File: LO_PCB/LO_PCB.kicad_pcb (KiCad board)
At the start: 4 copper layers, 50 x 44 mm, 97 parts, among them J1 PWR, J2 Conn_01x06, Q1 AO3401A, U1 TPS7A9101DSKT, U2 LMX2582RHAR, X1 TB612-100.0M

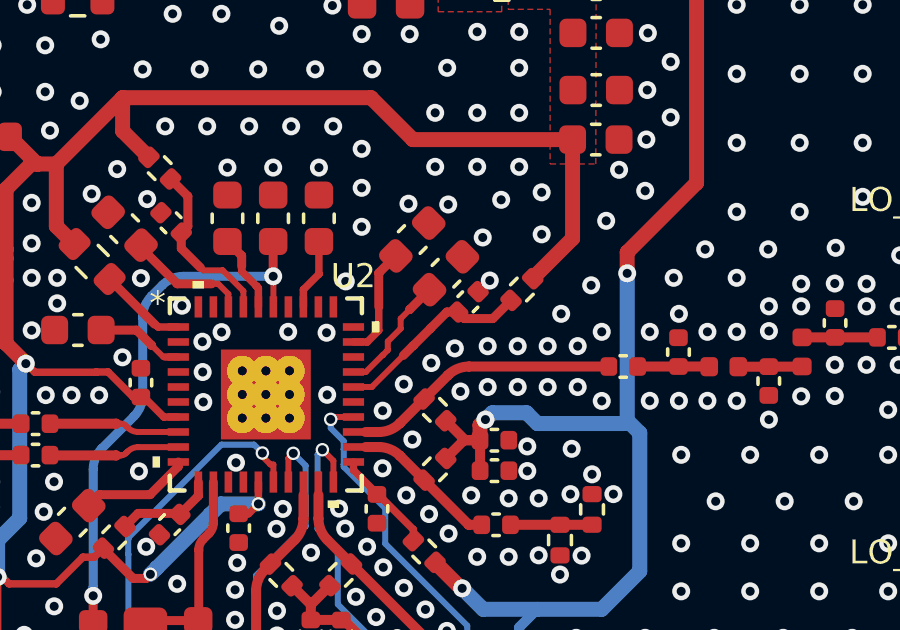
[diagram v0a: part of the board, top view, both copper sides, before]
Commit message: fixed errors and small bugs
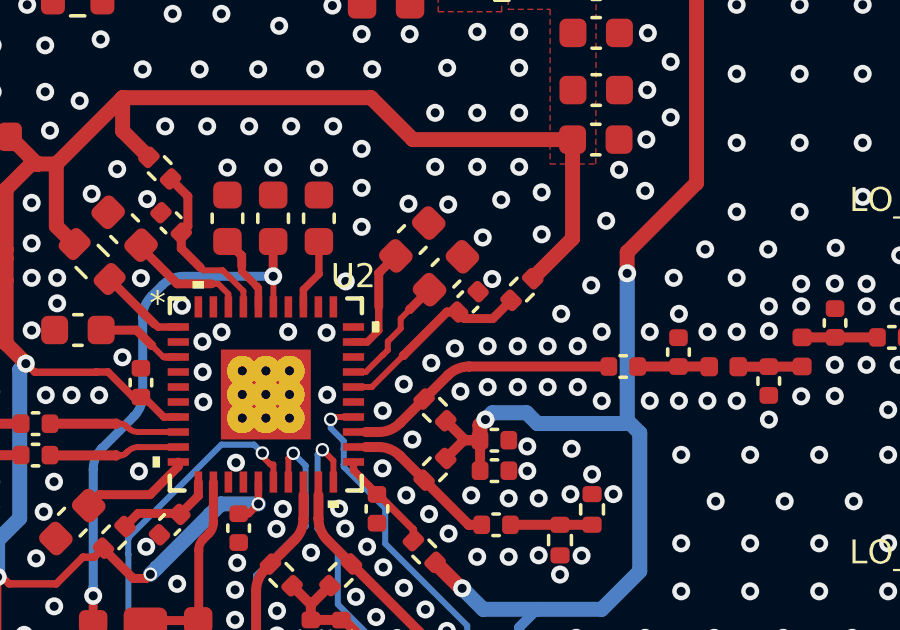
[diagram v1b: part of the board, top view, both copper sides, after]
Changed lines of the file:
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@@
 	)
 	(via
-		(at 165.02 94.69)
+		(at 165.1 94.6404)
 		(size 0.6)
 		(drill 0.3)
@@
 	)
 	(segment
-		(start 162.35 95.657092)
-		(end 163.011992 94.9951)
-		(width 0.3)
-		(layer "F.Cu")
-		(net "Net-(U2-VBIASVCO2)")
-	)
-	(segment
-		(start 162.05 96.292092)
-		(end 161.62 96.722092)
+		(start 161.62 97.01)
+		(end 161.455 97.175)
 		(width 0.2)
 		(layer "F.Cu")
@@
 	)
 	(segment
-		(start 160.886201 97.738799)
-		(end 160.476201 97.738799)
+		(start 161.45 97.175)
+		(end 160.886201 97.738799)
 		(width 0.2)
 		(layer "F.Cu")
@@
 	)
 	(segment
-		(start 161.62 97.01)
-		(end 161.455 97.175)
-		(width 0.2)
+		(start 162.35 95.66)
+		(end 162.35 95.657092)
+		(width 0.3)
 		(layer "F.Cu")
 		(net "Net-(U2-VBIASVCO2)")
 	)
 	(segment
-		(start 163.168446 95.1651)
-		(end 163.176992 95.1651)
-		(width 0.25)
+		(start 162.05 96.292092)
+		(end 161.62 96.722092)
+		(width 0.2)
 		(layer "F.Cu")
 		(net "Net-(U2-VBIASVCO2)")
 	)
 	(segment
-		(start 162.35 95.65)
-		(end 162.35 95.66)
+		(start 160.886201 97.738799)
+		(end 160.476201 97.738799)
 		(width 0.2)
 		(layer "F.Cu")
@@
 	)
 	(segment
-		(start 163.153982 95.1401)
-		(end 163.130621 95.1401)
+		(start 163.168446 95.1651)
+		(end 163.176992 95.1651)
 		(width 0.25)
 		(layer "F.Cu")
@@
 	)
 	(segment
-		(start 161.62 96.722092)
-		(end 161.62 97.01)
-		(width 0.2)
+		(start 163.153982 95.1401)
+		(end 163.130621 95.1401)
+		(width 0.25)
 		(layer "F.Cu")
 		(net "Net-(U2-VBIASVCO2)")
 	)
 	(segment
-		(start 162.35 95.66)
-		(end 162.35 95.657092)
+		(start 162.35 95.657092)
+		(end 163.011992 94.9951)
 		(width 0.3)
 		(layer "F.Cu")
@@
 	)
 	(segment
-		(start 162.05 95.96)
-		(end 162.05 96.292092)
+		(start 161.62 96.722092)
+		(end 161.62 97.01)
 		(width 0.2)
 		(layer "F.Cu")
@@
 	)
 	(segment
-		(start 161.45 97.175)
-		(end 160.886201 97.738799)
+		(start 162.05 95.96)
+		(end 162.05 96.292092)
 		(width 0.2)
 		(layer "F.Cu")
@@
 	)
 	(segment
-		(start 162.138117 97.188117)
-		(end 162.461335 96.8649)
-		(width 0.3)
-		(layer "F.Cu")
-		(net "Net-(U2-VCCVCO2)")
-	)
-	(segment
-		(start 162.4649 96.8649)
-		(end 163.05 96.2798)
-		(width 0.3)
-		(layer "F.Cu")
-		(net "Net-(U2-VCCVCO2)")
-	)
-	(segment
 		(start 161.087435 98.2388)
 		(end 160.476201 98.2388)
@@
 	)
 	(segment
-		(start 162.461335 96.8649)
-		(end 162.4649 96.8649)
+		(start 162.138117 97.188117)
+		(end 162.141883 97.188117)
 		(width 0.3)
 		(layer "F.Cu")
@@
 	)
 	(segment
-		(start 163.05 96.2798)
-		(end 163.0502 96.2798)
-		(width 0.3)
-		(layer "F.Cu")
-		(net "Net-(U2-VCCVCO2)")
-	)
-	(segment
-		(start 165.121386 95.958614)
-		(end 165.729375 95.350625)
+		(start 162.141883 97.188117)
+		(end 163.590589 95.739411)
 		(width 0.3)
 		(layer "F.Cu")
@@
 	)
 	(segment
-		(start 163.0502 96.2798)
-		(end 163.590589 95.739411)
+		(start 165.121386 95.958614)
+		(end 165.729375 95.350625)
 		(width 0.3)
 		(layer "F.Cu")
